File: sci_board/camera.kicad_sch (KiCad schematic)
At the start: 7 parts, among them J3 10051922-2410EHLF

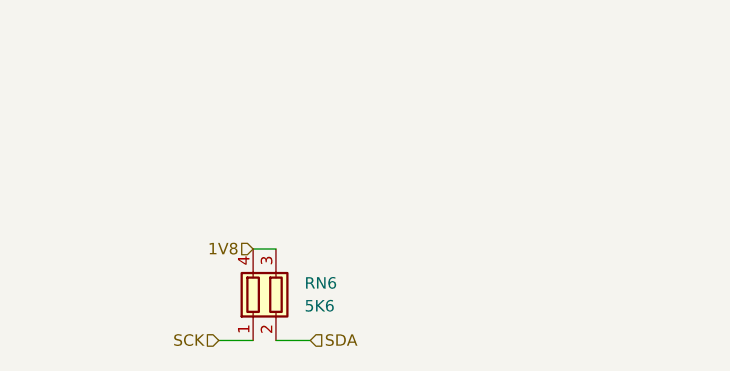
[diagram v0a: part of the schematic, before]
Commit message: power traces and vias of AUX and SCIlite are 0,5mm and 0.5/1.0mm
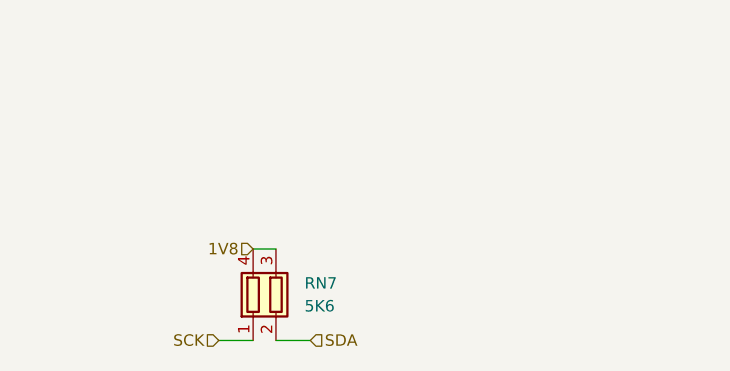
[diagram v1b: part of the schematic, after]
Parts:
- renumbered RN6 to RN7
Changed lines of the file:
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@@
 		(dnp no)
 		(fields_autoplaced yes)
-		(property "Reference" "RN6"
+		(property "Reference" "RN7"
 			(at 48.26 104.7749 0)
 			(effects
@@
 			(project "sci_board_wo_switches"
 				(path "/b4b2c88d-f6cd-4e60-862d-e21f68728580/5e5b27f8-7a4c-45d0-95f8-aff71797fcd3/21d0e59e-a5df-4633-9634-c7d789255f22"
-					(reference "RN6")
+					(reference "RN7")
 					(unit 1)
 				)
 				(path "/b4b2c88d-f6cd-4e60-862d-e21f68728580/5e5b27f8-7a4c-45d0-95f8-aff71797fcd3/3e22df28-91f0-4c0f-b958-7bfd7fe99c70"
-					(reference "RN7")
+					(reference "RN8")
 					(unit 1)
 				)
 				(path "/b4b2c88d-f6cd-4e60-862d-e21f68728580/5e5b27f8-7a4c-45d0-95f8-aff71797fcd3/87e2c931-24b0-464d-a54c-5e253d37e662"
-					(reference "RN8")
+					(reference "RN9")
 					(unit 1)
 				)

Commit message: EPS needs flash to self update with bootloader
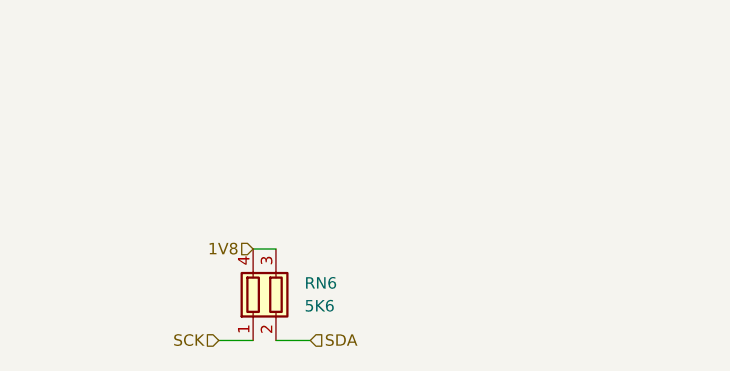
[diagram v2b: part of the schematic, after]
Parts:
- renumbered RN7 to RN6
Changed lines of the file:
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@@
 		(dnp no)
 		(fields_autoplaced yes)
-		(property "Reference" "RN7"
+		(property "Reference" "RN6"
 			(at 48.26 104.7749 0)
 			(effects
@@
 			(project "sci_board_wo_switches"
 				(path "/b4b2c88d-f6cd-4e60-862d-e21f68728580/5e5b27f8-7a4c-45d0-95f8-aff71797fcd3/21d0e59e-a5df-4633-9634-c7d789255f22"
+					(reference "RN6")
+					(unit 1)
+				)
+				(path "/b4b2c88d-f6cd-4e60-862d-e21f68728580/5e5b27f8-7a4c-45d0-95f8-aff71797fcd3/3e22df28-91f0-4c0f-b958-7bfd7fe99c70"
 					(reference "RN7")
 					(unit 1)
 				)
-				(path "/b4b2c88d-f6cd-4e60-862d-e21f68728580/5e5b27f8-7a4c-45d0-95f8-aff71797fcd3/3e22df28-91f0-4c0f-b958-7bfd7fe99c70"
+				(path "/b4b2c88d-f6cd-4e60-862d-e21f68728580/5e5b27f8-7a4c-45d0-95f8-aff71797fcd3/87e2c931-24b0-464d-a54c-5e253d37e662"
 					(reference "RN8")
 					(unit 1)
 				)
-				(path "/b4b2c88d-f6cd-4e60-862d-e21f68728580/5e5b27f8-7a4c-45d0-95f8-aff71797fcd3/87e2c931-24b0-464d-a54c-5e253d37e662"
-					(reference "RN9")
-					(unit 1)
-				)

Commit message: move project to new location, update sympbol, footprint and step paths
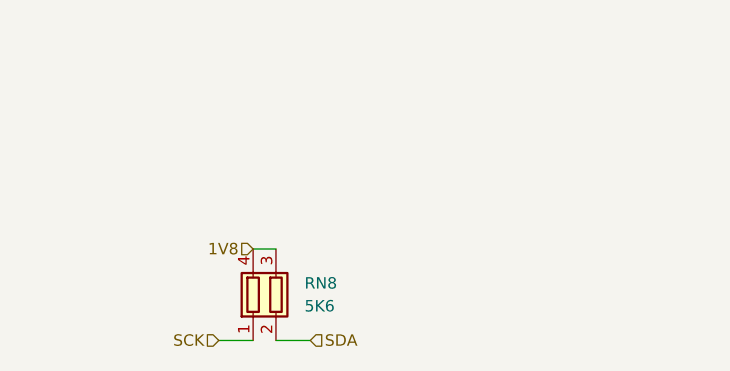
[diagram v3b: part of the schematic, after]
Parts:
- renumbered RN6 to RN8
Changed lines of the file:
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@@
 		(dnp no)
 		(fields_autoplaced yes)
-		(property "Reference" "RN6"
+		(property "Reference" "RN8"
 			(at 48.26 104.7749 0)
 			(effects
@@
 			(project "sci_board_wo_switches"
 				(path "/b4b2c88d-f6cd-4e60-862d-e21f68728580/5e5b27f8-7a4c-45d0-95f8-aff71797fcd3/21d0e59e-a5df-4633-9634-c7d789255f22"
-					(reference "RN6")
+					(reference "RN8")
 					(unit 1)
 				)
 				(path "/b4b2c88d-f6cd-4e60-862d-e21f68728580/5e5b27f8-7a4c-45d0-95f8-aff71797fcd3/3e22df28-91f0-4c0f-b958-7bfd7fe99c70"
-					(reference "RN7")
+					(reference "RN9")
 					(unit 1)
 				)
 				(path "/b4b2c88d-f6cd-4e60-862d-e21f68728580/5e5b27f8-7a4c-45d0-95f8-aff71797fcd3/87e2c931-24b0-464d-a54c-5e253d37e662"
-					(reference "RN8")
+					(reference "RN10")
 					(unit 1)
 				)

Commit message: VRef+ meeds to be connected to VDDA, should not be left floating
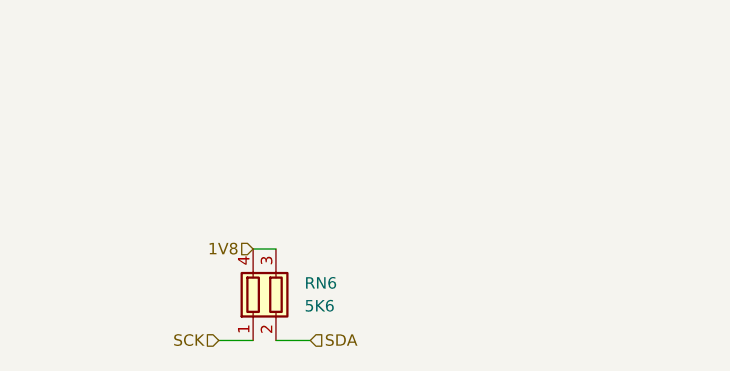
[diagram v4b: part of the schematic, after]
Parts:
- renumbered RN8 to RN6
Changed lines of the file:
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@@
 		(dnp no)
 		(fields_autoplaced yes)
-		(property "Reference" "RN8"
+		(property "Reference" "RN6"
 			(at 48.26 104.7749 0)
 			(effects
@@
 			(project "sci_board_wo_switches"
 				(path "/b4b2c88d-f6cd-4e60-862d-e21f68728580/5e5b27f8-7a4c-45d0-95f8-aff71797fcd3/21d0e59e-a5df-4633-9634-c7d789255f22"
+					(reference "RN6")
+					(unit 1)
+				)
+				(path "/b4b2c88d-f6cd-4e60-862d-e21f68728580/5e5b27f8-7a4c-45d0-95f8-aff71797fcd3/3e22df28-91f0-4c0f-b958-7bfd7fe99c70"
+					(reference "RN7")
+					(unit 1)
+				)
+				(path "/b4b2c88d-f6cd-4e60-862d-e21f68728580/5e5b27f8-7a4c-45d0-95f8-aff71797fcd3/87e2c931-24b0-464d-a54c-5e253d37e662"
 					(reference "RN8")
 					(unit 1)
 				)
-				(path "/b4b2c88d-f6cd-4e60-862d-e21f68728580/5e5b27f8-7a4c-45d0-95f8-aff71797fcd3/3e22df28-91f0-4c0f-b958-7bfd7fe99c70"
-					(reference "RN9")
-					(unit 1)
-				)
-				(path "/b4b2c88d-f6cd-4e60-862d-e21f68728580/5e5b27f8-7a4c-45d0-95f8-aff71797fcd3/87e2c931-24b0-464d-a54c-5e253d37e662"
-					(reference "RN10")
-					(unit 1)
-				)
